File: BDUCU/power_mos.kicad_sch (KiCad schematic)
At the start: 10 parts, among them Q1 MMBT3906, Q2 BSC019N04LS

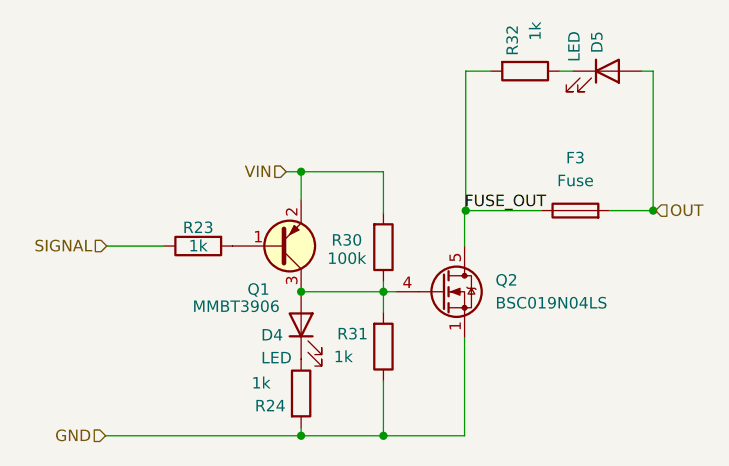
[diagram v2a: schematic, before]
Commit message: bducu scheme done, waiting for check
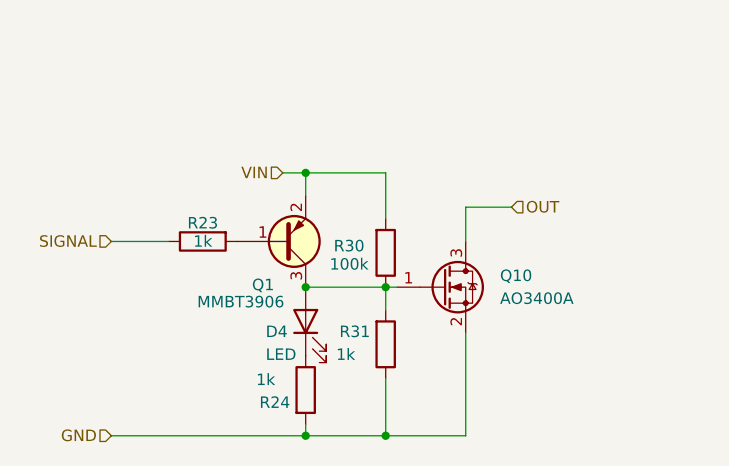
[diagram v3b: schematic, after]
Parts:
- removed D5: LED, RMC_LED:LED_0805_2012Metric_Pad1.45x1.40mm_HandSolder, symbol Device:LED
- removed F3: Fuse, RMC_Connnector:3 in 1 fuseholder, symbol Device:Fuse
- removed Q2: BSC019N04LS, RMC_SO:Infineon_PG-TDSON-8_6.15x5.15mm, symbol Transistor_FET:BSC061N08NS5
- removed R32: 1k, RMC_Resistor:R_0805_2012Metric_Pad1.20x1.40mm_HandSolder_L, symbol Device:R
- added Q10: AO3400A, RMC_SOT:SOT-23, symbol Transistor_FET:AO3400A
- Q1: footprint Better_Handsolder:SOT-23 -> RMC_SOT:SOT-23
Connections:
- net GND: now also Q10.2 (S)
- net OUT: now also Q10.3 (D)
- net at D4.2 (A), Q1.3 (C), R30.1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: now also Q10.1 (G)
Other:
- moved on the sheet: D4, Q1, R23, R24, R30
